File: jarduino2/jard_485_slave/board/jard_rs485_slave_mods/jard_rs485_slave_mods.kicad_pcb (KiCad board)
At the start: 2 copper layers, 81 x 66 mm, 24 parts, among them J1 NETWORK IN, J2 NETWORK OUT, J4 LED, J5 Niveau bas, J6 Electrovanne 12V, J7 Niveau Haut, Q1 TIP41C, U1 BPC_Mod485

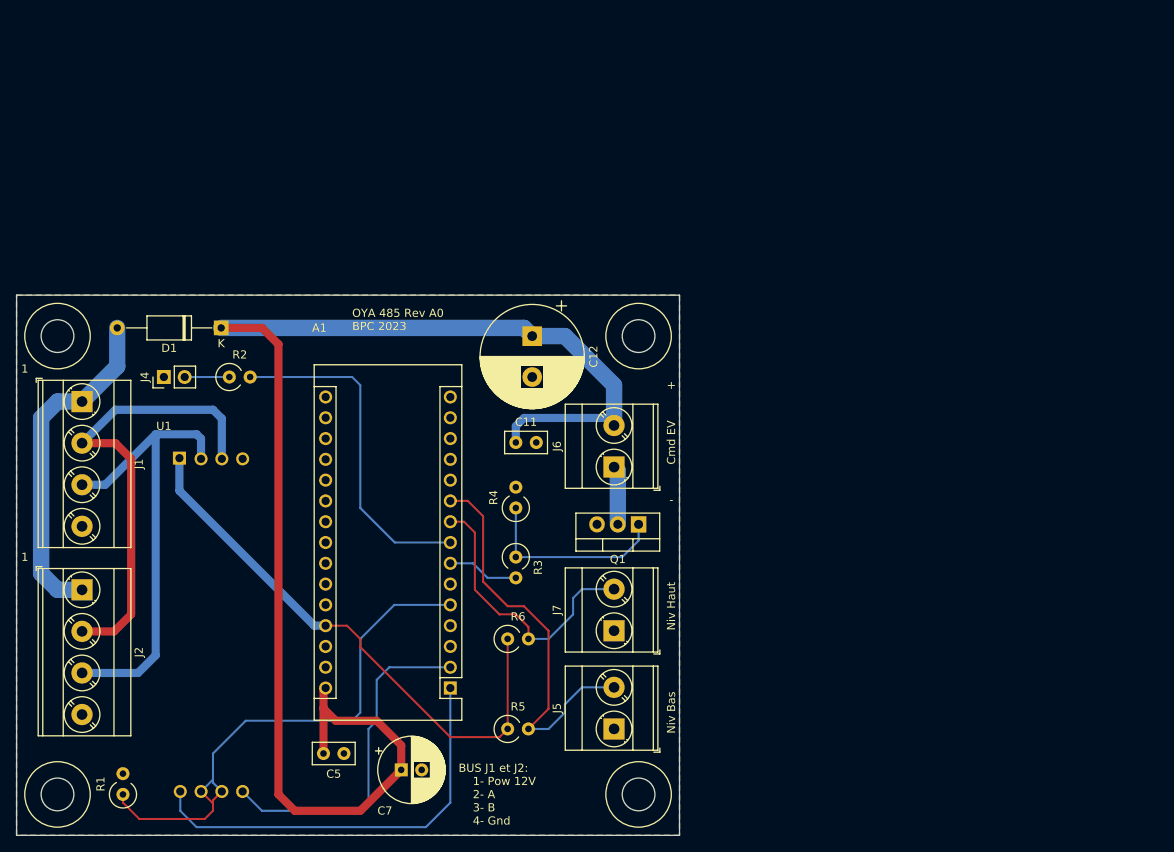
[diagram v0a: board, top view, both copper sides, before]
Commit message: Carte en L
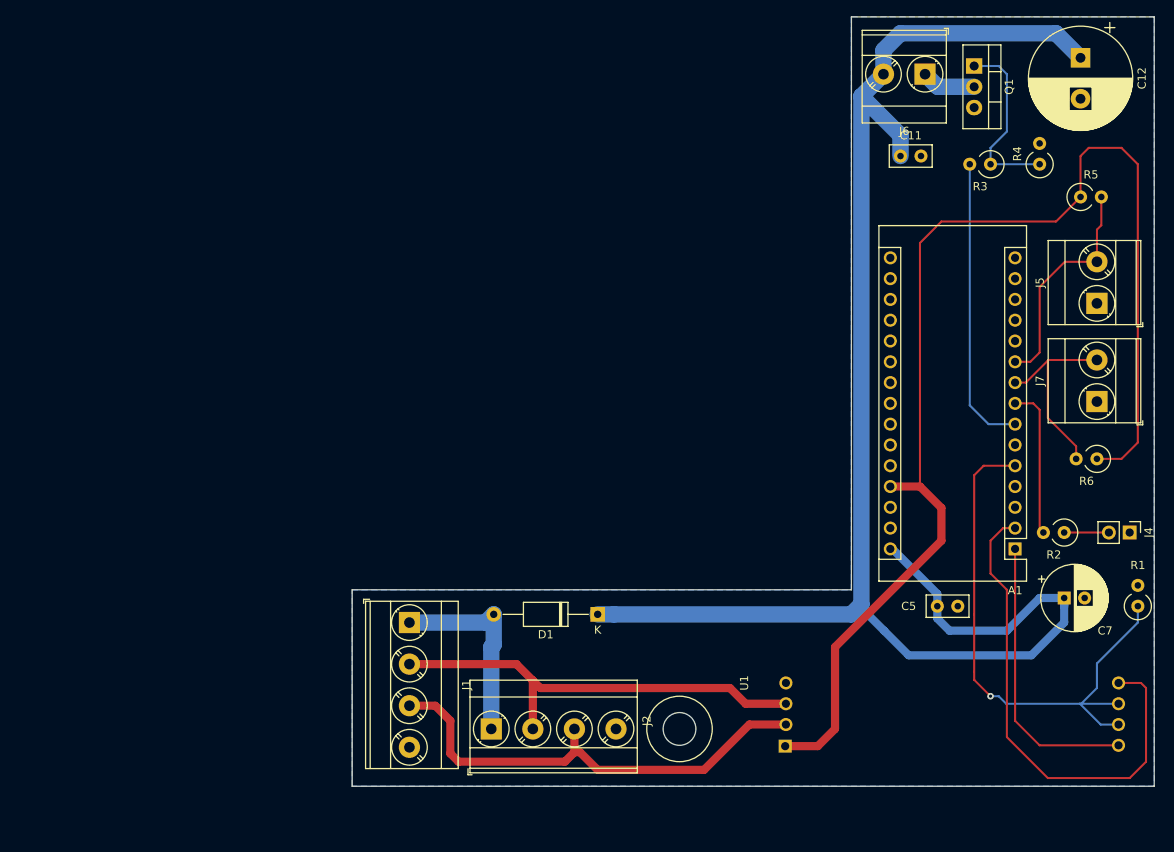
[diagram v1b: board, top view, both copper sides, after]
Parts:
- removed the REF** at (136.0, 125.0)
- removed the REF** at (136.0, 69.0)
- removed the REF** at (65.0, 125.0)
- removed the REF** at (65.0, 69.0)
- added REF**: BPC_Trou4mm_Fixation, bpc:BPC_Trou4mm_Fixation, F.Cu at (141.0, 117.0)
- moved R1 126.1 mm to (197.0, 102.0)
- moved J4 119.5 mm to (196.0, 93.0), turned to 270 degrees
- moved R2 103.8 mm to (188.0, 93.0), turned to 180 degrees
- moved R5 95.5 mm to (190.0, 52.0)
- moved C7 83.7 mm to (188.0, 101.0)
- moved U1 81.9 mm to (154.0, 119.0), turned to 90 degrees
- moved J5 78.6 mm to (192.0, 65.0)
- moved C5 77.1 mm to (175.0, 102.0)
- moved R4 76.6 mm to (185.0, 48.0)
- moved R3 75.3 mm to (179.0, 48.0), turned to 180 degrees
- moved R6 75.3 mm to (192.0, 84.0), turned to 180 degrees
- moved C12 75.1 mm to (190.0, 35.0)
- moved A1 71.1 mm to (182.0, 95.0)
- moved Q1 69.4 mm to (177.0, 36.0), turned to 270 degrees
- moved J7 65.3 mm to (192.0, 77.0)
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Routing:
- net Vcc: track 68.6 -> 151.4 mm
- net CMD_EV: track 8.74 -> 36.0 mm
- net Net-(A1-Pad30): track 173.8 -> 199.5 mm
- net Net-(A1-Pad8): track 41.6 -> 18.5 mm
- net IN_LVL_LOW: track 49.4 -> 27.9 mm
- net RX: track 41.8 -> 61.0 mm
- net Net-(D1-Pad2): track 41.4 -> 24.8 mm
- net TX: track 51.4 -> 34.9 mm
- net IN_LVL_HIGH: track 34.6 -> 24.7 mm
- net Net-(J1-Pad2): track 56.8 -> 53.9 mm
- net TXEN: track 67.1 -> 69.9 mm, vias 0 -> 1
- net Net-(Q1-Pad1): track 23.8 -> 22.2 mm
- net Net-(J1-Pad3): track 56.7 -> 57.7 mm
- net Net-(J6-Pad1): track 7.19 -> 6.64 mm
- removed copper zone on F.Cu, net GND
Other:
- board size 81 x 66 mm -> 98 x 94 mm
- board text removed: "+"
- board text removed: "-"
- board text removed: "1"
- board text removed: "BUS J1 et J2: 1- Pow 12V 2- A 3- B 4- Gnd"
- board text removed: "Cmd EV"
- board text removed: "Niv Bas"
- board text removed: "Niv Haut"
- board text removed: "OYA 485 Rev A0 BPC 2023"

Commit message: ?
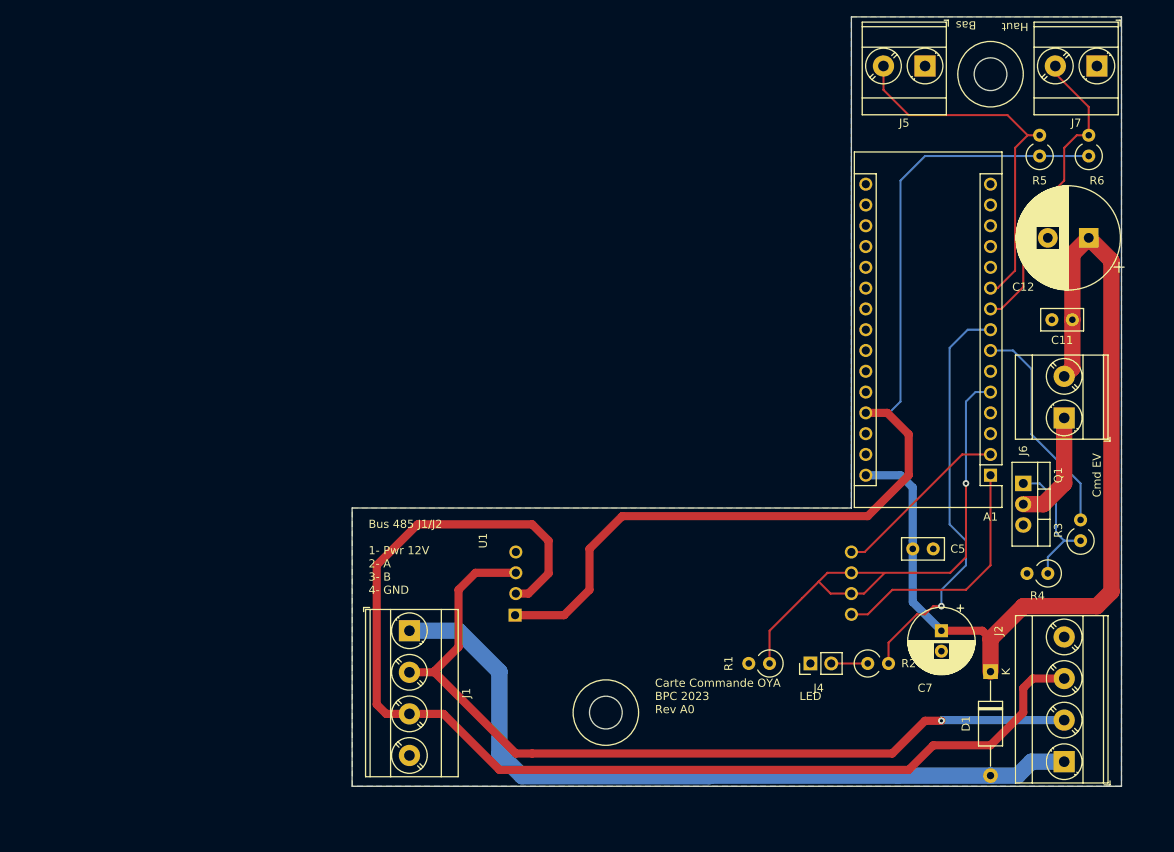
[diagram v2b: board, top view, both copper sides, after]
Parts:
- added REF**: BPC_Trou4mm_Fixation, bpc:BPC_Trou4mm_Fixation, F.Cu at (179.0, 37.0)
- U1: value BPC_Mod485 -> Arduino_Mod_RS485
- moved J2 70.1 mm to (188.0, 121.0), turned to 90 degrees
- moved Q1 51.4 mm to (183.0, 87.0)
- moved R4 50.0 mm to (186.0, 98.0), turned to 180 degrees
- moved D1 48.5 mm to (179.0, 110.0), turned to 270 degrees
- moved R3 47.3 mm to (190.0, 94.0), turned to 90 degrees
- moved R1 45.5 mm to (152.0, 109.0), turned to 180 degrees
- moved J6 45.3 mm to (188.0, 79.0), turned to 90 degrees
- moved J4 42.2 mm to (157.0, 109.0), turned to 90 degrees
- moved J7 41.0 mm to (192.0, 36.0), turned to 180 degrees
- moved R6 37.0 mm to (191.0, 47.0), turned to 90 degrees
- moved U1 36.7 mm to (121.0, 103.0)
- moved J5 35.8 mm to (171.0, 36.0), turned to 180 degrees
- moved C11 29.0 mm to (189.0, 67.0), turned to 180 degrees
- moved R2 28.8 mm to (164.0, 109.0), turned to 0 degrees
- moved C12 22.0 mm to (191.0, 57.0), turned to 180 degrees
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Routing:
- net Net-(J1-Pad3): track 57.7 -> 143.6 mm
- net Net-(A1-Pad30): track 199.5 -> 115.4 mm
- net Net-(D1-Pad2): track 24.8 -> 94.0 mm
- net Net-(J1-Pad2): track 53.9 -> 105.0 mm, vias 0 -> 1
- net RX: track 61.0 -> 22.3 mm
- net Net-(A1-Pad8): track 18.5 -> 50.4 mm, vias 0 -> 1
- net Vcc: track 151.4 -> 125.5 mm
- net IN_LVL_LOW: track 27.9 -> 45.6 mm
- net IN_LVL_HIGH: track 24.7 -> 38.0 mm
- net CMD_EV: track 36.0 -> 26.9 mm
- net Net-(J6-Pad1): track 6.64 -> 14.1 mm
- net TXEN: track 69.9 -> 63.8 mm
- net Net-(Q1-Pad1): track 22.2 -> 17.1 mm
- net TX: track 34.9 -> 30.8 mm
- net Net-(J4-Pad2): track 5.46 -> 4.46 mm
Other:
- board size 98 x 94 mm -> 94 x 94 mm
- board text added: "Bas"
- board text added: "Bus 485 J1/J2 1- Pwr 12V 2- A 3- B 4- GND"
- board text added: "Carte Commande OYA BPC 2023 Rev A0"
- board text added: "Cmd EV"
- board text added: "Haut"
- board text added: "LED"
